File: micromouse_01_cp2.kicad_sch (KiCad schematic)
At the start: 30 parts, among them IC1 MPU-6500, IC2 DRV8835DSSR, M1 MK06-4.5, M2 MK06-4.5, U1 MA730, U2 MA730, U3 ESP32-S3-PICO-1-N8R2

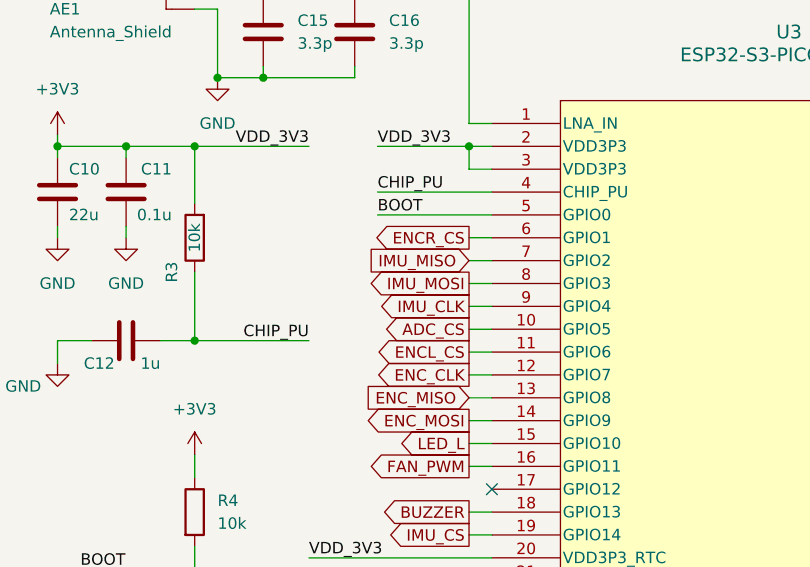
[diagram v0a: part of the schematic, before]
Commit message: 新しい部品乗せた
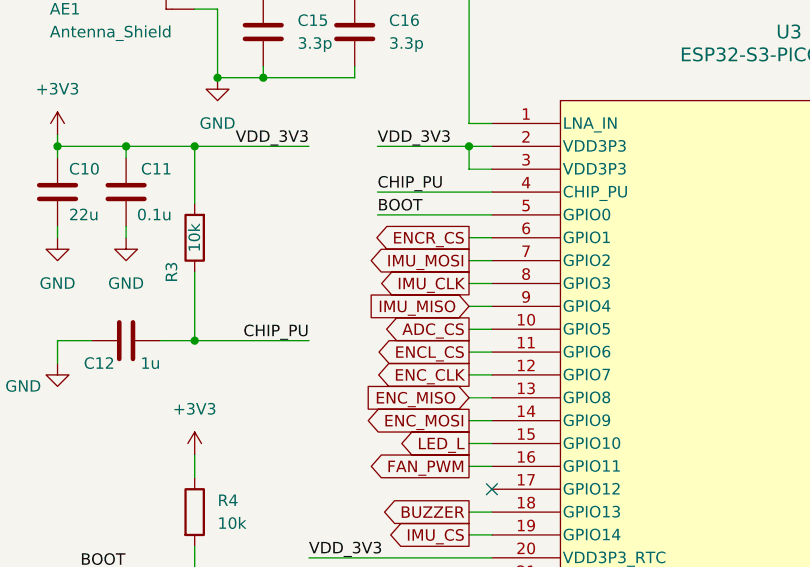
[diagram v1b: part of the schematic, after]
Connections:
- net IMU_CLK: now also U3.8 (GPIO3); no longer U3.9 (GPIO4)
- net IMU_MISO: now also U3.9 (GPIO4); no longer U3.7 (GPIO2)
- net IMU_MOSI: now also U3.7 (GPIO2); no longer U3.8 (GPIO3)
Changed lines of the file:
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@@
     )
   )
-  (global_label "IMU_MOSI" (shape output) (at 187.96 50.8 180) (fields_autoplaced)
+  (global_label "IMU_MISO" (shape input) (at 187.96 53.34 180) (fields_autoplaced)
     (effects (font (size 1.27 1.27)) (justify right))
-    (property "Intersheetrefs" "${INTERSHEET_REFS}" (at 176.0243 50.8 0)
+    (property "Intersheetrefs" "${INTERSHEET_REFS}" (at 176.0243 53.34 0)
       (effects (font (size 1.27 1.27)) (justify right) hide)
     )
@@
     )
   )
-  (global_label "IMU_CLK" (shape output) (at 187.96 53.34 180) (fields_autoplaced)
-    (effects (font (size 1.27 1.27)) (justify right))
-    (property "Intersheetrefs" "${INTERSHEET_REFS}" (at 177.0524 53.34 0)
-      (effects (font (size 1.27 1.27)) (justify right) hide)
-    )
-  )
   (global_label "MOT_MODE" (shape input) (at 130.81 175.26 0) (fields_autoplaced)
     (effects (font (size 1.27 1.27)) (justify left))
     (property "Intersheetrefs" "${INTERSHEET_REFS}" (at 143.7132 175.26 0)
       (effects (font (size 1.27 1.27)) (justify left) hide)
+    )
+  )
+  (global_label "IMU_CLK" (shape output) (at 187.96 50.8 180) (fields_autoplaced)
+    (effects (font (size 1.27 1.27)) (justify right))
+    (property "Intersheetrefs" "${INTERSHEET_REFS}" (at 177.0524 50.8 0)
+      (effects (font (size 1.27 1.27)) (justify right) hide)
     )
   )
@@
     )
   )
-  (global_label "IMU_MISO" (shape input) (at 187.96 48.26 180) (fields_autoplaced)
-    (effects (font (size 1.27 1.27)) (justify right))
-    (property "Intersheetrefs" "${INTERSHEET_REFS}" (at 176.0243 48.26 0)
-      (effects (font (size 1.27 1.27)) (justify right) hide)
-    )
-  )
   (global_label "USB_D-" (shape bidirectional) (at 187.96 93.98 180) (fields_autoplaced)
     (effects (font (size 1.27 1.27)) (justify right))
@@
     )
   )
+  (global_label "IMU_MOSI" (shape output) (at 187.96 48.26 180) (fields_autoplaced)
+    (effects (font (size 1.27 1.27)) (justify right))
+    (property "Intersheetrefs" "${INTERSHEET_REFS}" (at 176.0243 48.26 0)
+      (effects (font (size 1.27 1.27)) (justify right) hide)
+    )
+  )

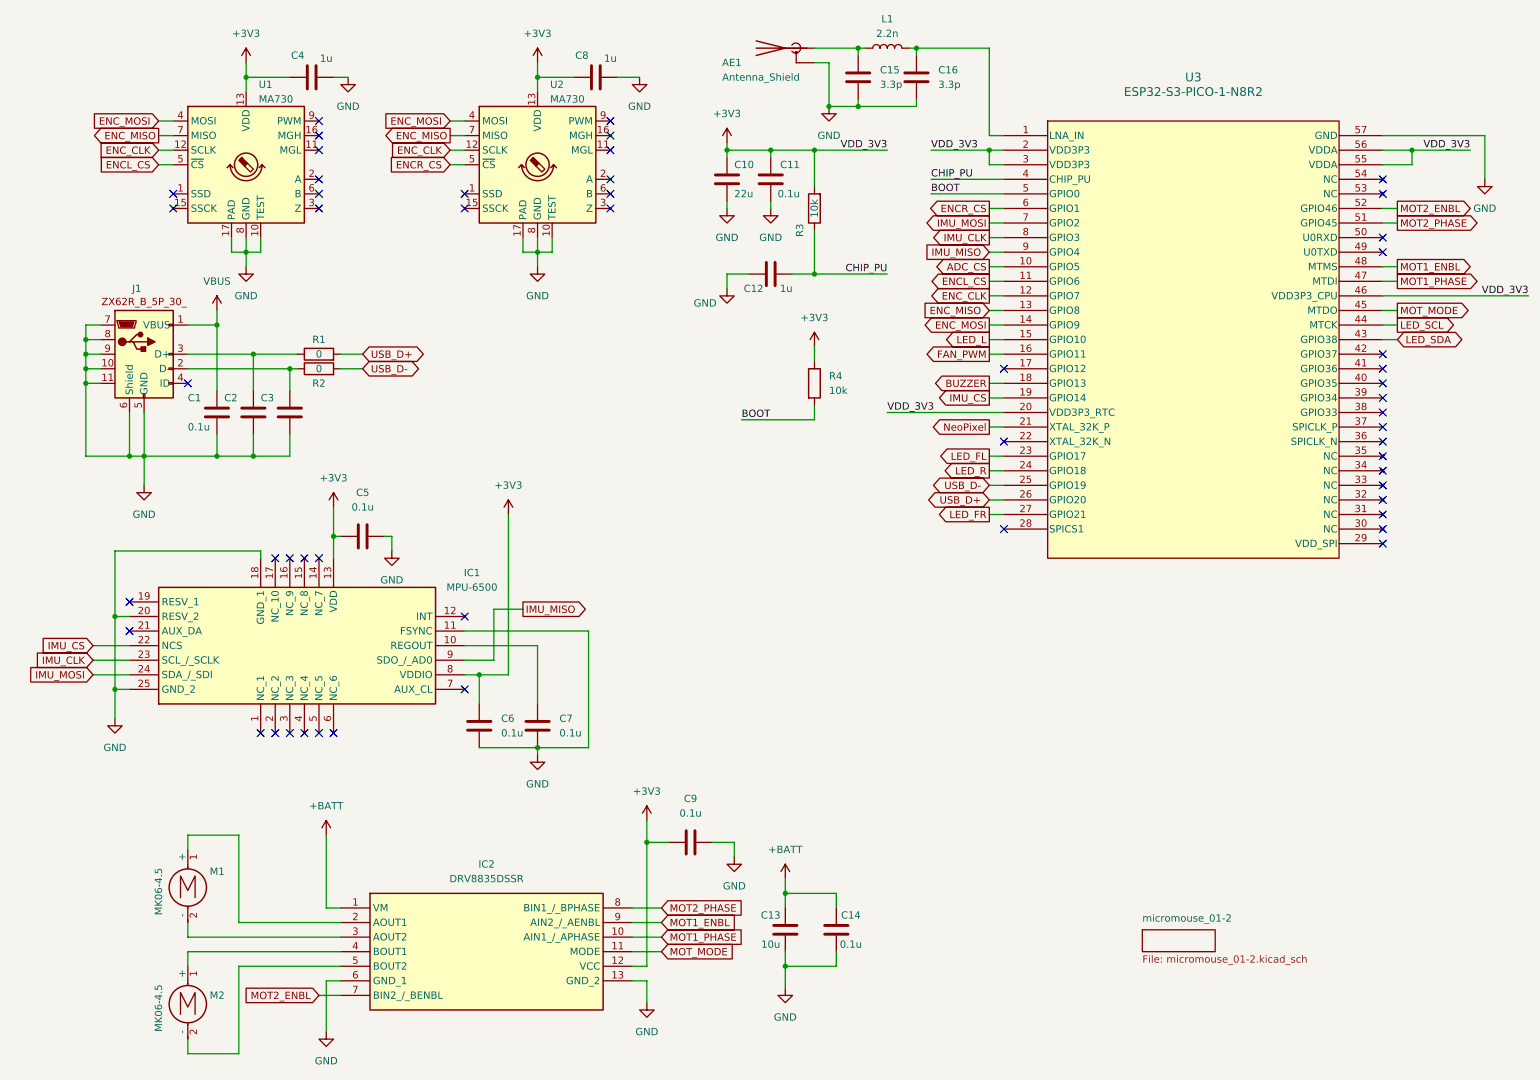
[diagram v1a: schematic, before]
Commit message: Initial Commit
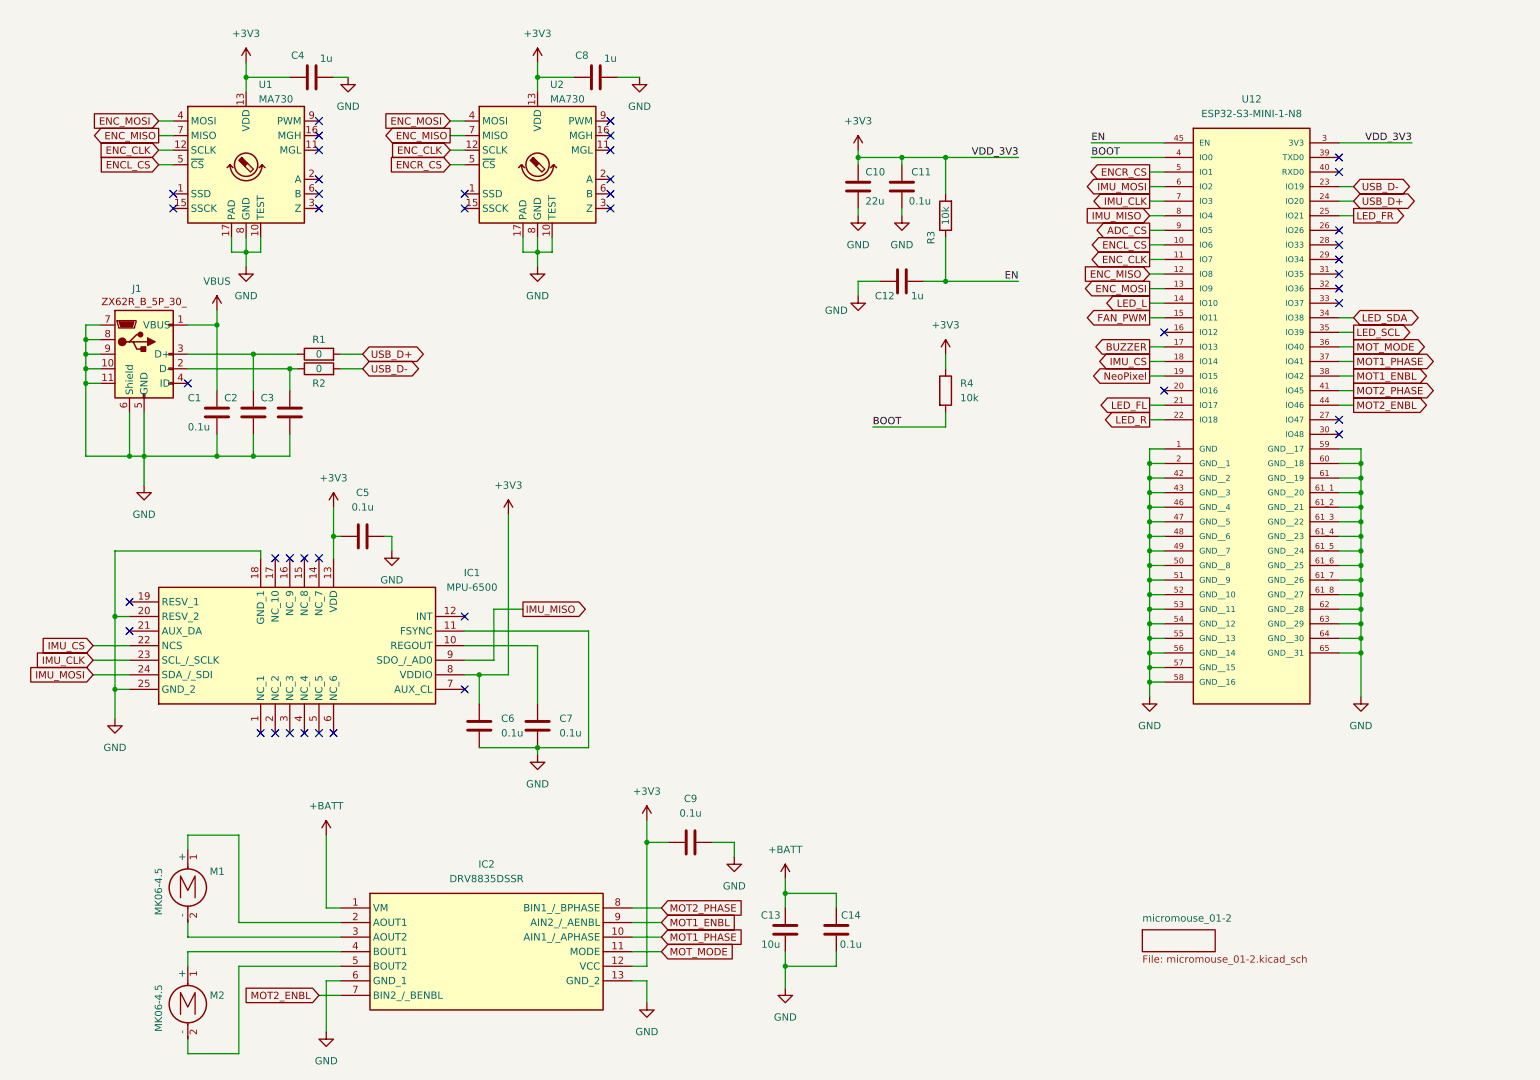
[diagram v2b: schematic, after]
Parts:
- removed AE1: Antenna_Shield, RF_Antenna:Texas_SWRA117D_2.4GHz_Right, symbol Device:Antenna_Shield
- removed C15, C16: 3.3p, Capacitor_SMD:C_0402_1005Metric, symbol Device:C
- removed L1: 2.2n, Inductor_SMD:L_0402_1005Metric, symbol Device:L
- removed U3: ESP32-S3-PICO-1-N8R2, QFN56_7X7_EXP, symbol 2024-02-29_13-39-39:ESP32-S3-PICO-1-N8R2
- added U12: ESP32-S3-MINI-1-N8, footprints:XCVR_ESP32-S3-MINI-1-N8, symbol ESP32-S3-MINI-1-N8:ESP32-S3-MINI-1-N8
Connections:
- net +3V3: now also U12.3 (3V3)
- net ADC_CS: now also U12.9 (IO5)
- net BOOT: now also U12.4 (IO0)
- net BUZZER: now also U12.17 (IO13)
- net ENCL_CS: now also U12.10 (IO6)
- net ENCR_CS: now also U12.5 (IO1)
- net ENC_CLK: now also U12.11 (IO7)
- net ENC_MISO: now also U12.12 (IO8)
- net ENC_MOSI: now also U12.13 (IO9)
- net FAN_PWM: now also U12.15 (IO11)
- net GND: now also U12.1 (GND), U12.2 (GND__1), U12.42 (GND__2), U12.43 (GND__3), U12.46 (GND__4), U12.47 (GND__5), U12.48 (GND__6), U12.49 (GND__7), U12.50 (GND__8), U12.51 (GND__9), U12.52 (GND__10), U12.53 (GND__11), U12.54 (GND__12), U12.55 (GND__13), U12.56 (GND__14), U12.57 (GND__15), U12.58 (GND__16), U12.59 (GND__17), U12.60 (GND__18), U12.61 (GND__19), U12.61_1 (GND__20), U12.61_2 (GND__21), U12.61_3 (GND__22), U12.61_4 (GND__23), U12.61_5 (GND__24), U12.61_6 (GND__25), U12.61_7 (GND__26), U12.61_8 (GND__27), U12.62 (GND__28), U12.63 (GND__29), U12.64 (GND__30), U12.65 (GND__31)
- net IMU_CLK: now also U12.7 (IO3)
- net IMU_CS: now also U12.18 (IO14)
- net IMU_MISO: now also U12.8 (IO4)
- net IMU_MOSI: now also U12.6 (IO2)
- net LED_FL: now also U12.21 (IO17)
- net LED_FR: now also U12.25 (IO21)
- net LED_L: now also U12.14 (IO10)
- net LED_R: now also U12.22 (IO18)
- net LED_SCL: now also U12.35 (IO39)
- net LED_SDA: now also U12.34 (IO38)
- net MOT1_ENBL: now also U12.38 (IO42)
- net MOT1_PHASE: now also U12.37 (IO41)
- net MOT2_ENBL: now also U12.44 (IO46)
- net MOT2_PHASE: now also U12.41 (IO45)
- net MOT_MODE: now also U12.36 (IO40)
- net NeoPixel: now also U12.19 (IO15)
- net USB_D+: now also U12.24 (IO20)
- net USB_D-: now also U12.23 (IO19)
- net CHIP_PU renamed EN
- net EN: now also U12.45 (EN)
- no-connect marks 52 -> 43
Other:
- moved on the sheet: C10, C11, C12, R3, R4
